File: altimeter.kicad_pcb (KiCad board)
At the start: 2 copper layers, 45 x 24 mm, 47 parts, among them J201 Conn_01x10, J202 Conn_ARM_JTAG_SWD_10, J203 Conn_02x03_Counter_Clockwise, J204 USB_B_Micro, J205 Conn_01x04, Q101 DMG2301L, Q301 BC847BDW1, Q401 BC847BDW1, Q501 BC847BDW1, U101 STM32F302CCTx, U102 MT25Q, U103 AIS2120SXTR, U104 MIC5219-3.3YM5, U105 LF50_TO252, U106 LM397, U107 MS5611-01BA, U301 SI7232DN, U501 SI7232DN, Y101 Crystal_Small

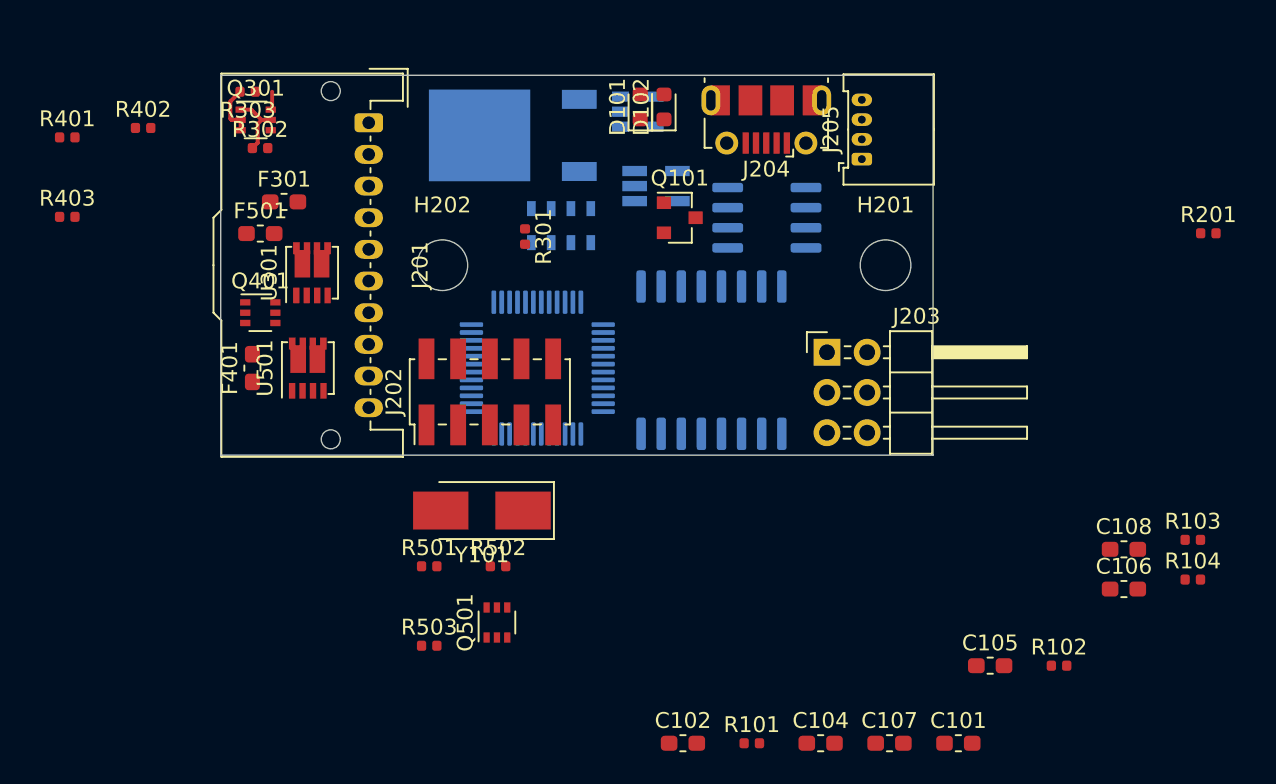
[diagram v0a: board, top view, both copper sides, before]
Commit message: update
Signed-off-by: Thomas Schmid <tom@lfence.de>
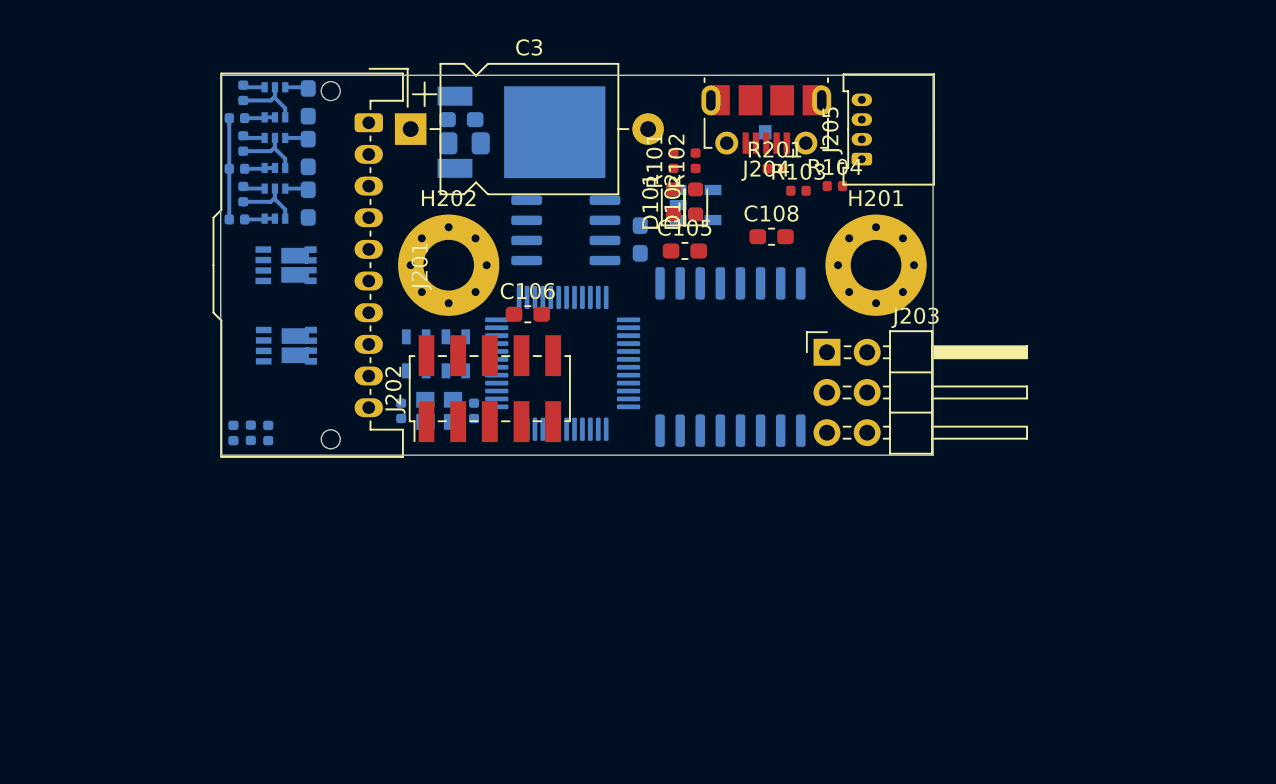
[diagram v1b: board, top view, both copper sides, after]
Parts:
- removed U106: LM397, Package_TO_SOT_SMD:SOT-23-5_HandSoldering
- removed Y101: Crystal_Small, Crystal:Crystal_SMD_5032-2Pin_5.0x3.2mm_HandSoldering
- added C103: 1u, Capacitor_SMD:C_0603_1608Metric_Pad1.05x0.95mm_HandSolder, B.Cu at (164.5, 107.4)
- added C3: CP, Capacitor_THT:CP_Axial_L11.0mm_D8.0mm_P15.00mm_Horizontal, F.Cu at (150.0, 100.4)
- added Y1: Crystal_GND24, Crystal:Crystal_SMD_2520-4Pin_2.5x2.0mm, B.Cu at (151.8, 118.2)
- C101, C102: footprint Capacitor_SMD:C_0603_1608Metric_Pad1.05x0.95mm_HandSolder -> Capacitor_SMD:C_0402_1005Metric; moved to B.Cu
- C104: footprint Capacitor_SMD:C_0603_1608Metric_Pad1.05x0.95mm_HandSolder -> Capacitor_SMD:C_0805_2012Metric_Pad1.15x1.40mm_HandSolder; moved to B.Cu
- C107, F301, F401, F501, Q101, Q301, Q401, Q501, R301, R302, R303, R401, R402, R403, R501, R502, R503, U301, U501: moved to B.Cu
- H201, H202: footprint MountingHole:MountingHole_3.2mm_M3_DIN965 -> MountingHole:MountingHole_3.2mm_M3_Pad_Via
- moved C107 47.8 mm to (153.2, 99.8)
- moved C104 44.1 mm to (153.4, 101.3)
- moved C106 41.5 mm to (157.4, 112.1)
- moved R102 39.3 mm to (168.0, 102.4), turned to 90 degrees
- moved R101 37.1 mm to (166.6, 102.4), turned to 90 degrees
- moved C101 37.1 mm to (154.0, 118.2), turned to 90 degrees
- moved R104 33.6 mm to (176.8, 104.0)
- moved R103 33.3 mm to (174.5, 104.3)
- moved C105 32.5 mm to (167.3, 108.1)
- moved Q501 29.9 mm to (141.4, 105.1)
- moved C108 29.8 mm to (172.8, 107.2)
- moved R503 29.5 mm to (139.0, 106.1)
- moved R502 28.5 mm to (139.4, 104.5), turned to 90 degrees
- moved R201 27.7 mm to (173.0, 102.9)
- moved C102 27.5 mm to (149.4, 118.2), turned to 270 degrees
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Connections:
- U301 pad 1: FIRE_PYRO1 -> FIRE_PYRO2
- U301 pad 3: FIRE_PYRO2 -> FIRE_PYRO1
- U301 pad 5: PYRO2_LOW -> PYRO1_LOW
- U301 pad 6: PYRO1_LOW -> PYRO2_LOW
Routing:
- net PYRO_TEST_ENABLE: track 0.00 -> 6.40 mm
- net Net-(Q501-Pad1): track 0.00 -> 4.28 mm
- net Net-(Q401-Pad1): track 0.00 -> 4.28 mm
- net GND: track 0.00 -> 4.22 mm
- net Net-(Q501-Pad2): track 0.00 -> 1.94 mm
- net Net-(Q401-Pad2): track 0.00 -> 1.94 mm
- net Net-(F501-Pad2): track 0.00 -> 1.48 mm
- net Net-(F401-Pad2): track 0.00 -> 1.48 mm
- net Net-(Q301-Pad2): track 3.29 -> 1.94 mm
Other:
- net class Default: clearance 0.2 -> 0.1651; trace_width 0.25 -> 0.1778
- rule trace_clearance: 0.2 -> 0.1651
- rule trace_min: 0.2 -> 0.1524
